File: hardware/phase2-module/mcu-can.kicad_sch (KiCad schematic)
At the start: 29 parts, among them J2 SWD, J3 UART, U10 STM32G431CBT6, U11 TCAN1042HGV, Y1 8MHz

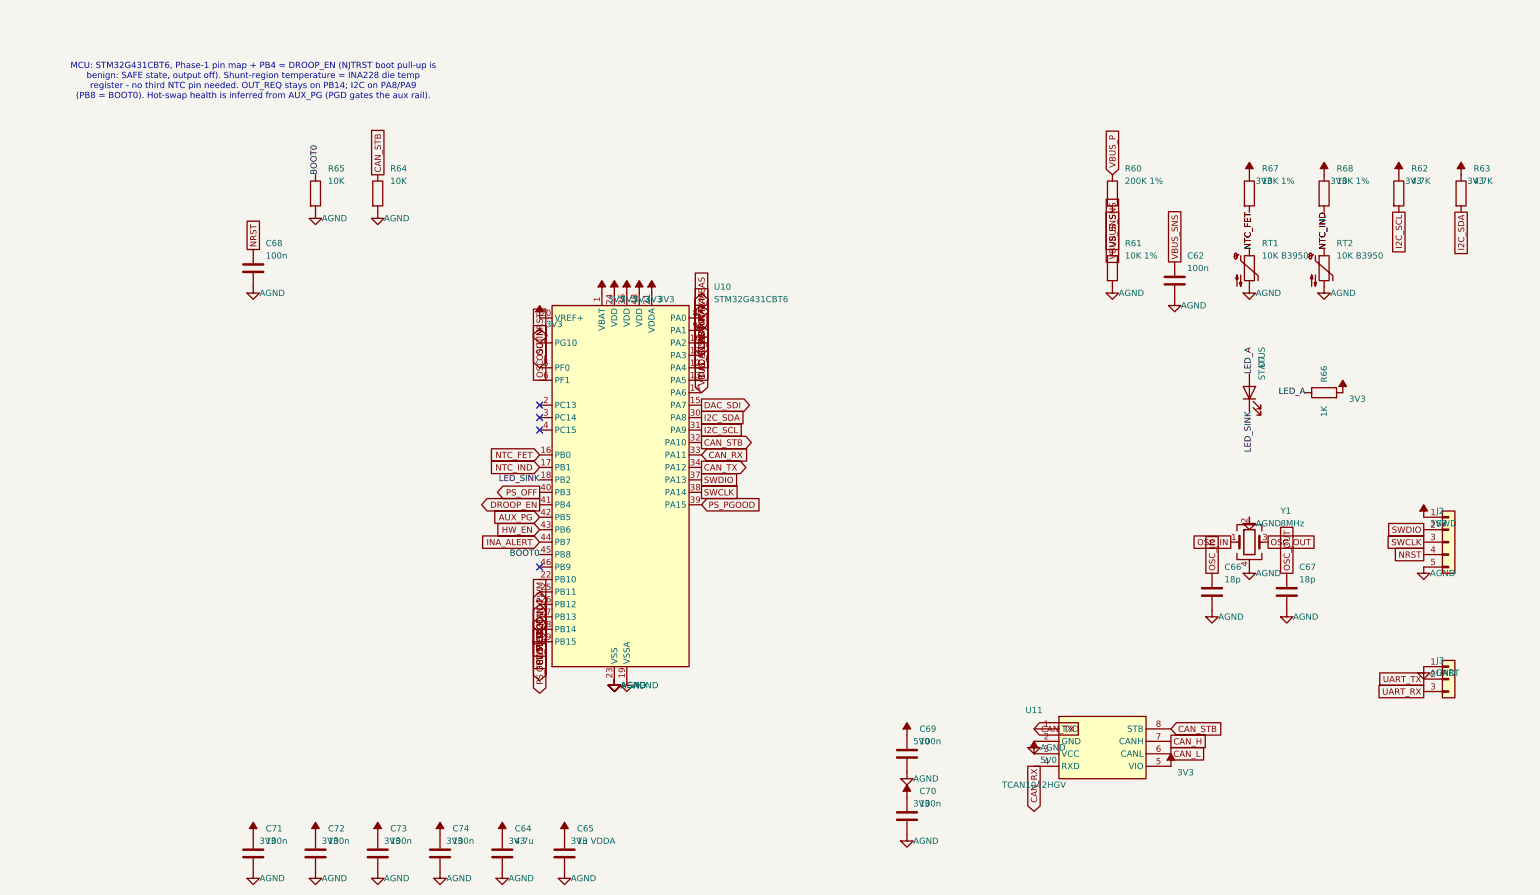
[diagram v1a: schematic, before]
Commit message: Refactor code structure for improved readability and maintainability
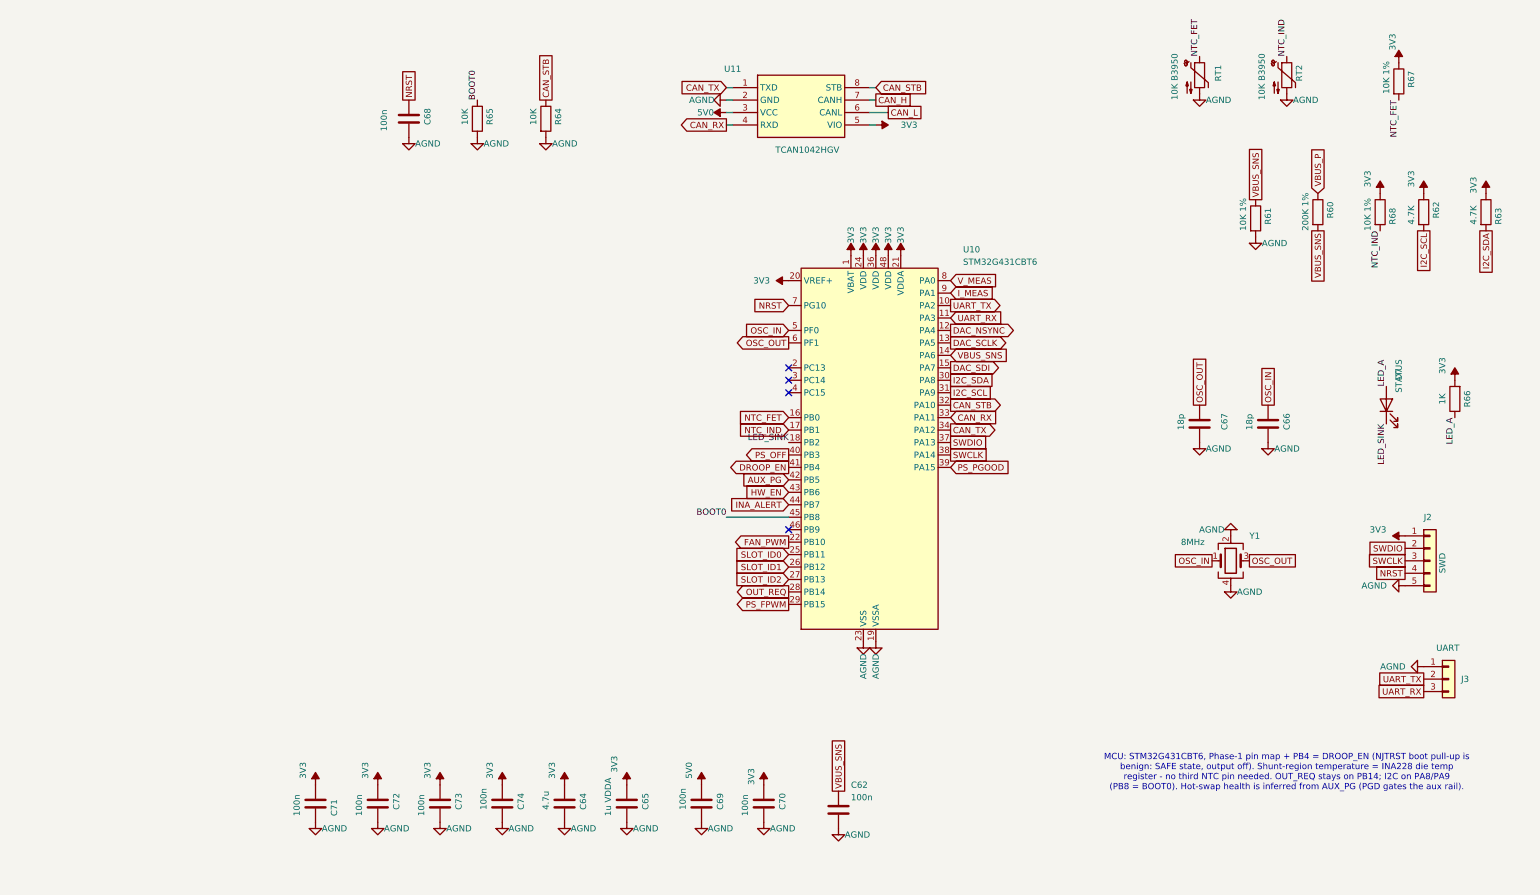
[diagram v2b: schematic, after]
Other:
- moved on the sheet: C62, C64, C65, C66, C67, C68, C69, C70, C71, C72, C73, C74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
